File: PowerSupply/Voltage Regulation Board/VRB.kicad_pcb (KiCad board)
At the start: 2 copper layers, 34.2 x 45.8 mm, 14 parts

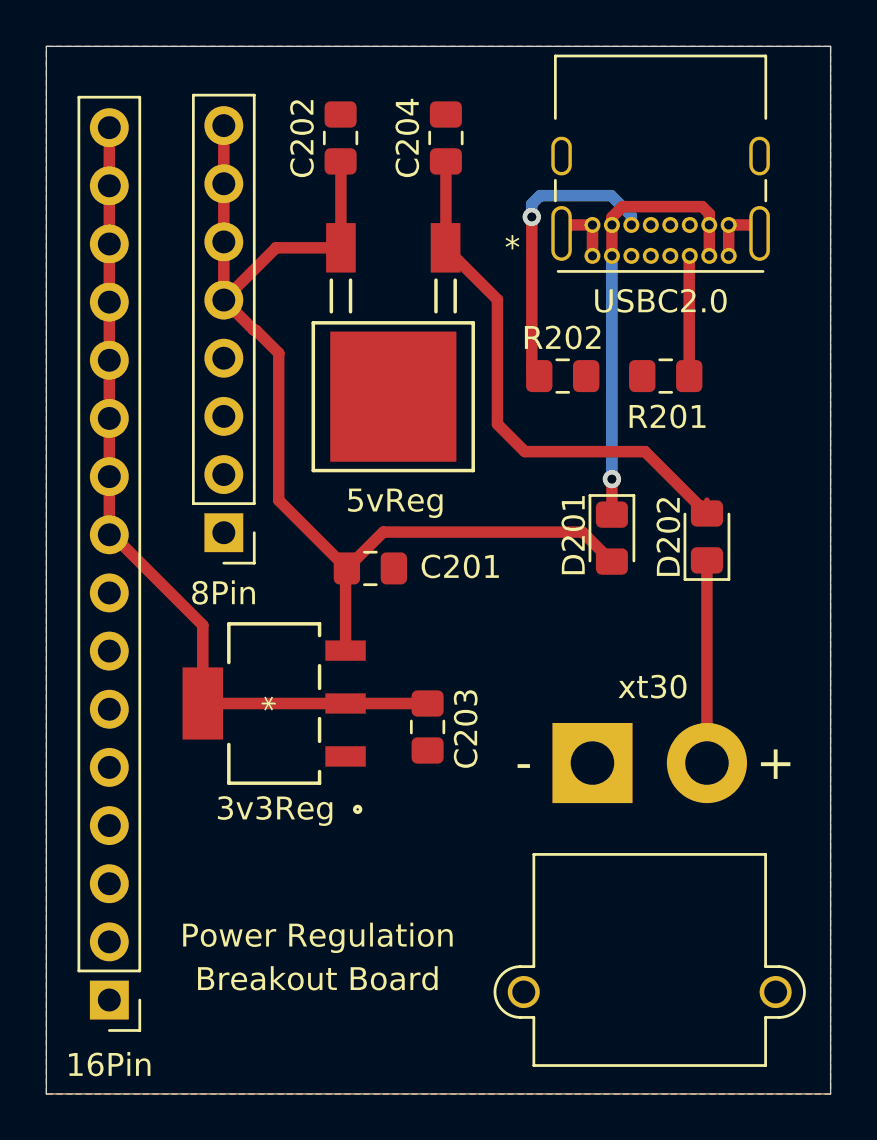
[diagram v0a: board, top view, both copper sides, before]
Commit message: Fixed Diode Thingy
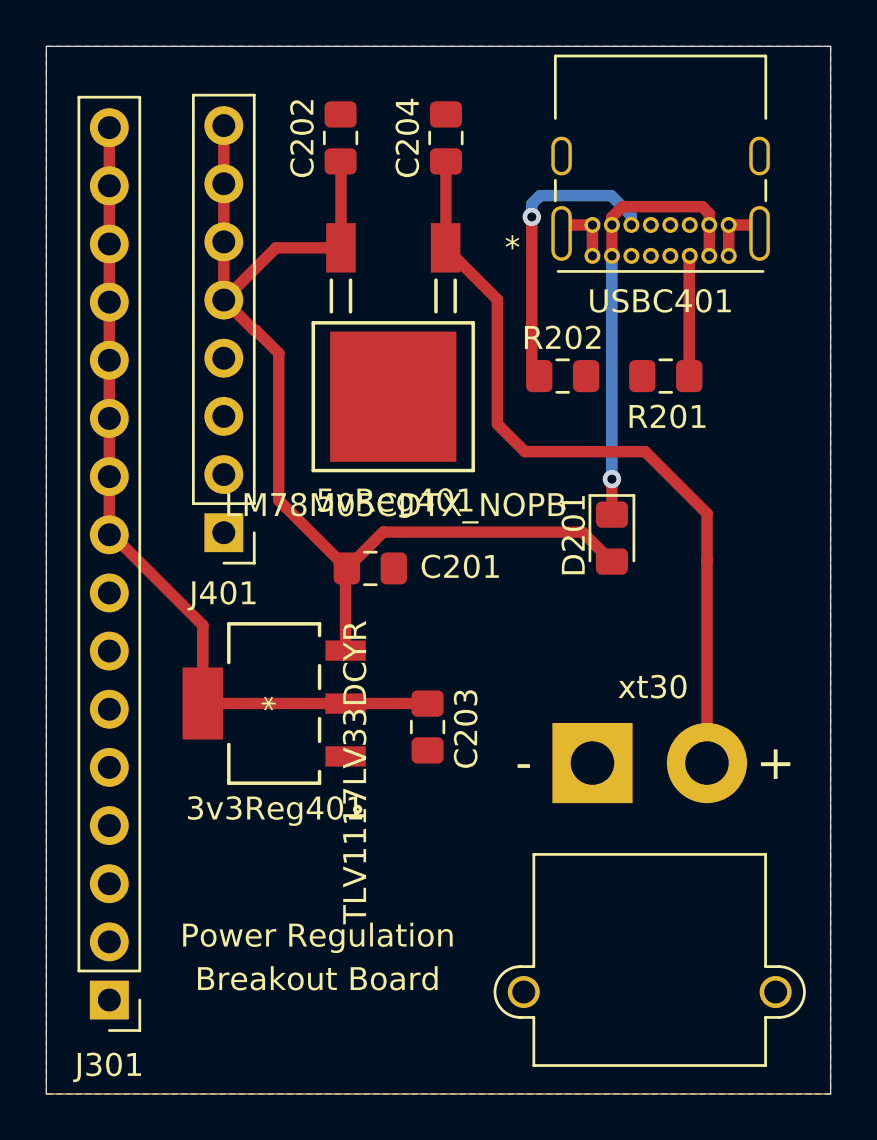
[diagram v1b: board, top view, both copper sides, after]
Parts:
- removed D202: DIODE, Diode_SMD:D_0805_2012Metric_Pad1.15x1.40mm_HandSolder
- 3v3Reg401: renamed from 3v3Reg; value (none) -> TLV1117LV33DCYR
- 5vReg401: renamed from 5vReg; value (none) -> LM78M05CDTX_NOPB
- renumbered 16Pin to J301, 8Pin to J401, USBC2.0 to USBC401
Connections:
- xt30 pad 2: Net-(D202-Pad1) -> Net-(5vReg401-Pad1)
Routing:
- net Net-(5vReg401-Pad1): track 23.8 -> 34.1 mm
- net Net-(D202-Pad1): track 8.85 -> 0.00 mm
